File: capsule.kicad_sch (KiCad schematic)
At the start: 89 parts, among them SW1 SW, SW10 SW, SW11 SW, SW12 SW, SW13 SW, SW14 SW, SW15 SW, SW16 SW, SW17 SW, SW18 SW, SW19 SW, SW2 SW, SW20 SW, SW21 SW, SW22 SW, SW23 SW, SW24 SW, SW25 SW, SW26 SW, SW27 SW, SW28 SW, SW29 SW, SW3 SW, SW30 SW, SW31 SW_Push, SW4 SW, SW5 SW, SW6 SW, SW7 SW, SW8 SW, SW9 SW, U2 ATmega32U4-A, Y1 16MHz

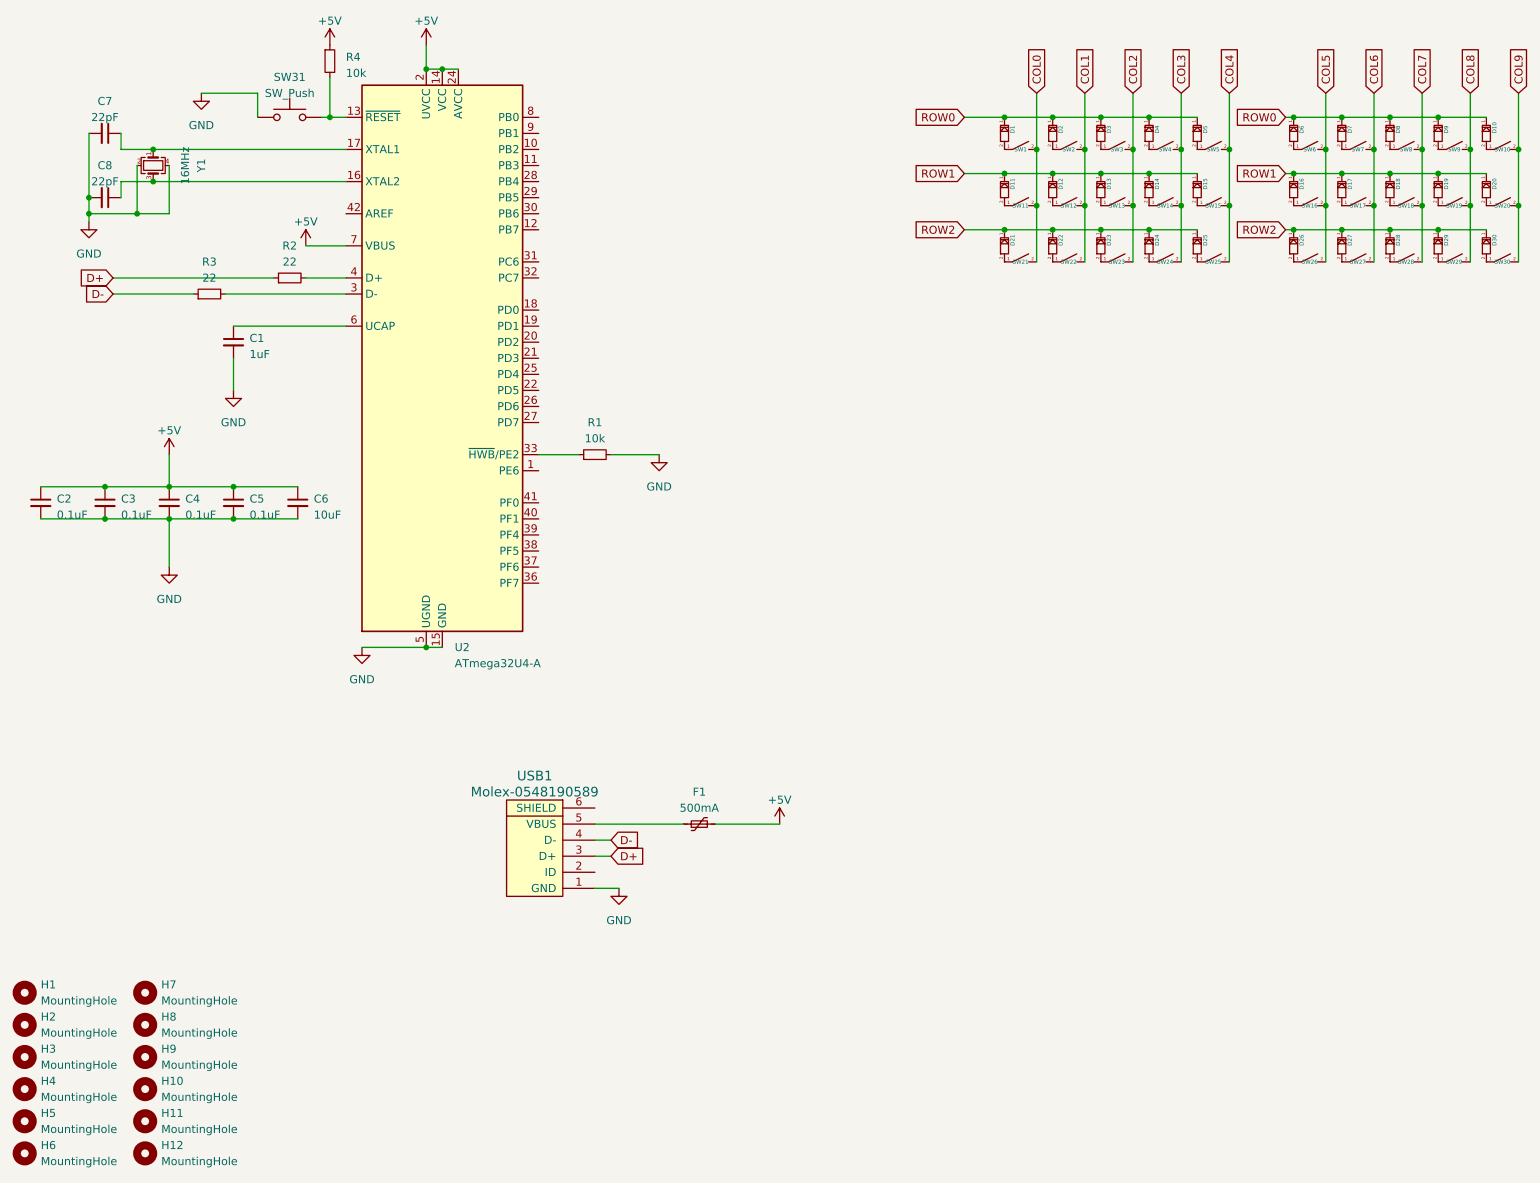
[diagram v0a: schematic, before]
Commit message: pcb refactor
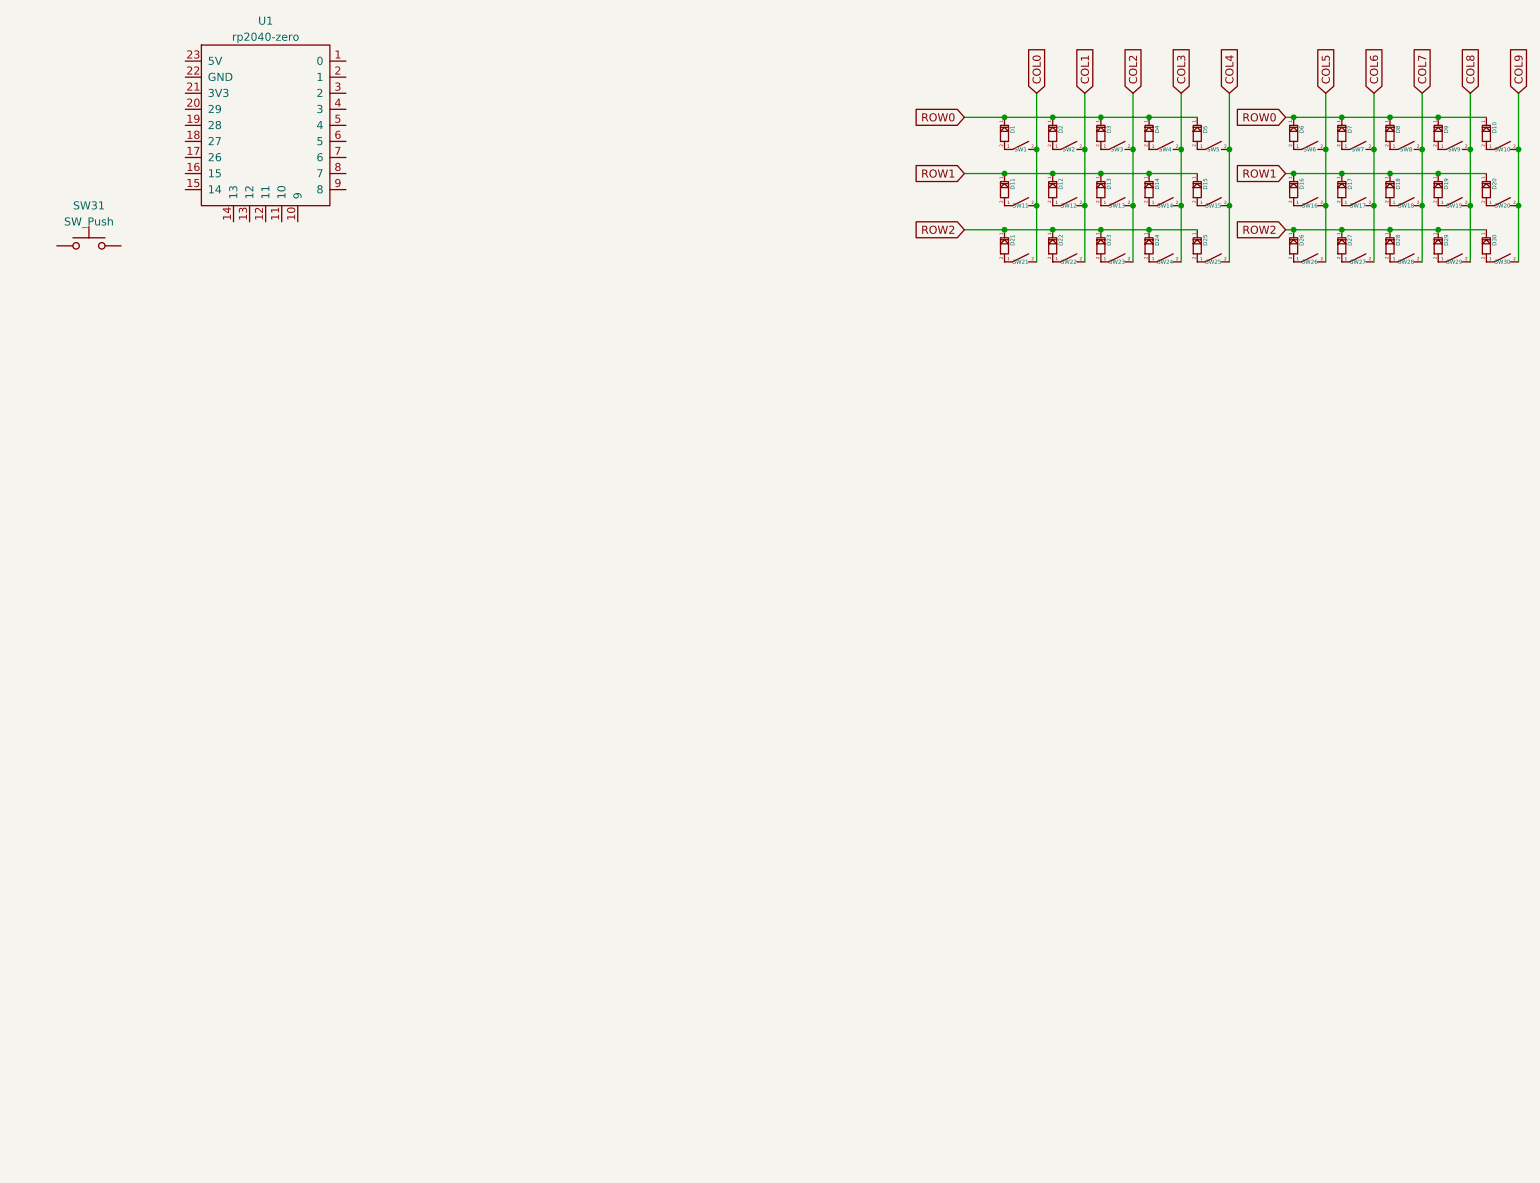
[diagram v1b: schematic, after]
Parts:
- removed C1: 1uF, Capacitor_SMD:C_0805_2012Metric, symbol Device:C_Small
- removed C2, C3, C4, C5: 0.1uF, Capacitor_SMD:C_0805_2012Metric, symbol Device:C_Small
- removed C6: 10uF, Capacitor_SMD:C_0805_2012Metric, symbol Device:C_Small
- removed C7, C8: 22pF, Capacitor_SMD:C_0805_2012Metric, symbol Device:C_Small
- removed F1: 500mA, Fuse:Fuse_1206_3216Metric, symbol Device:Polyfuse_Small
- removed H1, H10, H11, H12, H2, H3, H4, H5, H6, H7, H8, H9: MountingHole, MountingHole:MountingHole_3.2mm_M3_Pad_Via, symbol Mechanical:MountingHole
- removed R1, R4: 10k, Resistor_SMD:R_0805_2012Metric, symbol Device:R_Small
- removed R2, R3: 22, Resistor_SMD:R_0805_2012Metric, symbol Device:R_Small
- removed U2: ATmega32U4-A, Package_QFP:TQFP-44_10x10mm_P0.8mm, symbol MCU_Microchip_ATmega:ATmega32U4-A
- removed USB1: Molex-0548190589, random-keyboard-parts:Molex-0548190589, symbol random-keyboard-parts:Molex-0548190589
- removed Y1: 16MHz, Crystal:Crystal_SMD_3225-4Pin_3.2x2.5mm, symbol Device:Crystal_GND24_Small
- added U1: rp2040-zero, mcu:rp2040-zero-tht, symbol mcu:rp2040-zero
- SW1, SW10, SW11, SW12, SW13, SW14, SW15, SW16, SW17, SW18, SW19, SW2, SW20, SW21, SW22, SW23, SW24, SW25, SW26, SW27, SW28, SW29, SW3, SW30, SW4, SW5, SW6, SW7, SW8, SW9: footprint Kailh_Choc:KailhChoc-1U -> miketronic_fplib:MB_KailhChoc-1U
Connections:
- net GND: no longer names the net of SW31.1
